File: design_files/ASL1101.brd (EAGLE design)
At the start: 9.8 x 6.5 mm, 4 parts, among them SW1 KMT011

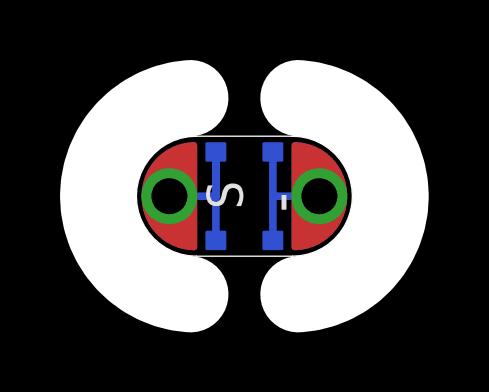
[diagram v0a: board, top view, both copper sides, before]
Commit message: update format
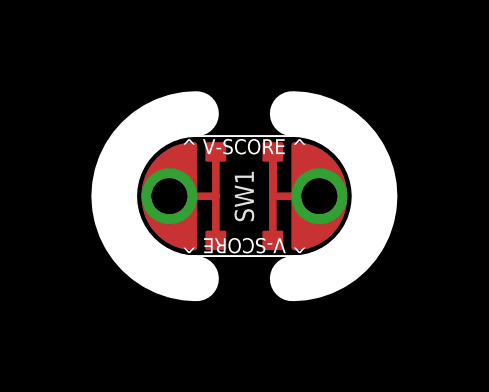
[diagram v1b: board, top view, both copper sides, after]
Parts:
- moved U$1 5.00 mm to (17.5, 20.0), flipped to the bottom
- moved U$7 5.00 mm to (22.5, 20.0), flipped to the bottom
- flipped SW1 to the top
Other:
- board size 9.8 x 6.5 mm -> 8.7 x 5.5 mm
- board text added: "2"
- board text added: "^ V-SCORE ^"
- board text removed: "1"
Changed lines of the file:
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@@
 <?xml version="1.0" encoding="utf-8"?>
 <!DOCTYPE eagle SYSTEM "eagle.dtd">
-<eagle version="6.2">
+<eagle version="6.3">
 <drawing>
 <settings>
@@
 <setting verticaltext="up"/>
 </settings>
-<grid distance="1" unitdist="mil" unit="mm" style="lines" multiple="1" display="yes" altdistance="0.025" altunitdist="inch" altunit="inch"/>
+<grid distance="1" unitdist="mm" unit="mm" style="lines" multiple="1" display="yes" altdistance="0.025" altunitdist="inch" altunit="inch"/>
 <layers>
 <layer number="1" name="Top" color="4" fill="1" visible="yes" active="yes"/>
@@
 <layer number="108" name="Dimension_circle" color="7" fill="1" visible="yes" active="yes"/>
 <layer number="109" name="Dimension_normal" color="7" fill="1" visible="yes" active="yes"/>
+<layer number="110" name="fp0" color="7" fill="1" visible="yes" active="yes"/>
 <layer number="111" name="tGTest" color="4" fill="1" visible="no" active="no"/>
 <layer number="112" name="bGTest" color="1" fill="1" visible="no" active="no"/>
@@
 <layer number="220" name="220bmp" color="7" fill="1" visible="yes" active="yes"/>
 <layer number="221" name="221bmp" color="7" fill="1" visible="yes" active="yes"/>
+<layer number="222" name="222bmp" color="7" fill="1" visible="yes" active="yes"/>
 <layer number="223" name="223bmp" color="7" fill="1" visible="yes" active="yes"/>
 <layer number="224" name="224bmp" color="7" fill="1" visible="yes" active="yes"/>
+<layer number="248" name="Housing" color="7" fill="1" visible="yes" active="yes"/>
+<layer number="249" name="Edge" color="7" fill="1" visible="yes" active="yes"/>
 <layer number="250" name="Descript" color="7" fill="1" visible="yes" active="yes"/>
 <layer number="251" name="SMDround" color="7" fill="1" visible="yes" active="yes"/>
@@
 <text x="48.111025" y="4.365003125" size="0.889" layer="48">TinyLily Switch - 3mm</text>
 <text x="44.986825" y="1.7714" size="0.889" layer="48">AS-PCB-ASL1101</text>
-<text x="67.3810375" y="1.6952" size="0.889" layer="48">1</text>
-<text x="21.884284375" y="19.46078125" size="1.5" layer="21" rot="R90">-</text>
-<text x="19.945059375" y="19.5675375" size="1.2" layer="21" rot="R90">S</text>
+<text x="67.3810375" y="1.6952" size="0.889" layer="48">2</text>
+<text x="18.115715625" y="19.46078125" size="1.5" layer="22" rot="MR90">-</text>
+<text x="20.054940625" y="19.5675375" size="1.2" layer="22" rot="MR90">S</text>
 <dimension x1="18" y1="22" x2="18" y2="18" x3="13.08319375" y3="20" layer="48"/>
 <text x="40.5384" y="14.481796875" size="0.4572" layer="48" ratio="10">Released under the Creative Commons Attribution Share-Alike 3.0 License</text>
@@
 <wire x1="18.4" y1="18" x2="18.4" y2="22" width="0.0254" layer="108" curve="-180"/>
 <wire x1="21.6" y1="22" x2="21.6" y2="18" width="0.0254" layer="108" curve="-180"/>
-<wire x1="18.2" y1="23.27" x2="18.2" y2="16.73" width="2.54" layer="46" curve="173"/>
-<wire x1="21.8" y1="16.73" x2="21.8" y2="23.27" width="2.54" layer="46" curve="173"/>
+<wire x1="18.4" y1="22.75" x2="18.4" y2="17.25" width="1.5" layer="46" curve="180"/>
+<wire x1="21.6" y1="17.25" x2="21.6" y2="22.75" width="1.5" layer="46" curve="180"/>
 <wire x1="18.4" y1="22" x2="21.6" y2="22" width="0.0254" layer="108"/>
 <wire x1="21.6" y1="18" x2="18.4" y2="18" width="0.0254" layer="109"/>
@@
 <wire x1="18.4" y1="22" x2="21.6" y2="22" width="0.0254" layer="20"/>
 <text x="40.5384" y="10.887796875" size="0.4572" layer="48" ratio="10">TinyDuino, TinyLily and TinyShield Designs by TinyCircuits</text>
+<wire x1="16.4" y1="22" x2="23.6" y2="22" width="0.0254" layer="20"/>
+<wire x1="23.6" y1="18" x2="16.4" y2="18" width="0.0254" layer="20"/>
+<text x="20" y="18.6" size="0.5" layer="20" rot="SR180" align="bottom-center">^ V-SCORE ^</text>
+<text x="20" y="21.4" size="0.5" layer="20" rot="SR0" align="bottom-center">^ V-SCORE ^</text>
 </plain>
 <attributes>
@@
 </class>
 </classes>
-<designrules>
+<designrules name="default">
 <description language="de">&lt;b&gt;EAGLE Design Rules&lt;/b&gt;
 &lt;p&gt;
@@
 <attribute name="NO_BOM" value="TRUE" x="44" y="0" size="1.778" layer="27" display="off"/>
 </element>
-<element name="U$1" library="tinycircuits" package="SEWTAP_TH_1206" value="SEWTABTH_1206" x="22.5" y="20" rot="R180">
-<attribute name="BOM" value="EXCLUDE" x="22.5" y="20" size="1.778" layer="27" rot="R180" display="off"/>
-<attribute name="DATABASE" value="./../../../../../Components/TinyCircuits_Part_Database.txt" x="22.5" y="20" size="1.778" layer="27" rot="R180" display="off"/>
-<attribute name="DNP" value="T" x="22.5" y="20" size="1.778" layer="27" rot="R180" display="off"/>
+<element name="U$1" library="tinycircuits" package="SEWTAP_TH_1206" value="SEWTABTH_1206" x="17.5" y="20" rot="MR180">
+<attribute name="BOM" value="EXCLUDE" x="17.5" y="20" size="1.778" layer="28" rot="MR180" display="off"/>
+<attribute name="DATABASE" value="./../../../../../Components/TinyCircuits_Part_Database.txt" x="17.5" y="20" size="1.778" layer="28" rot="MR180" display="off"/>
+<attribute name="DNP" value="T" x="17.5" y="20" size="1.778" layer="28" rot="MR180" display="off"/>
 </element>
-<element name="U$7" library="tinycircuits" package="SEWTAP_TH_1206" value="SEWTABTH_1206" x="17.5" y="20">
-<attribute name="BOM" value="EXCLUDE" x="17.5" y="20" size="1.778" layer="27" display="off"/>
-<attribute name="DATABASE" value="./../../../../../Components/TinyCircuits_Part_Database.txt" x="17.5" y="20" size="1.778" layer="27" display="off"/>
-<attribute name="DNP" value="T" x="17.5" y="20" size="1.778" layer="27" display="off"/>
+<element name="U$7" library="tinycircuits" package="SEWTAP_TH_1206" value="SEWTABTH_1206" x="22.5" y="20" rot="MR0">
+<attribute name="BOM" value="EXCLUDE" x="22.5" y="20" size="1.778" layer="28" rot="MR0" display="off"/>
+<attribute name="DATABASE" value="./../../../../../Components/TinyCircuits_Part_Database.txt" x="22.5" y="20" size="1.778" layer="28" rot="MR0" display="off"/>
+<attribute name="DNP" value="T" x="22.5" y="20" size="1.778" layer="28" rot="MR0" display="off"/>
 </element>
-<element name="SW1" library="tinycircuits" package="KMT011" value="KMT011" x="20" y="20" rot="MR90">
-<attribute name="PARTNO" value="AS-ITM-00041" x="20" y="20" size="1.778" layer="28" rot="MR90" display="off"/>
-<attribute name="VALUE" value="KMT011" x="20" y="20" size="1.778" layer="28" rot="MR90" display="off"/>
+<element name="SW1" library="tinycircuits" package="KMT011" value="KMT011" x="20" y="20" rot="R90">
+<attribute name="PARTNO" value="AS-ITM-00041" x="20" y="20" size="1.778" layer="27" rot="R90" display="off"/>
+<attribute name="VALUE" value="KMT011" x="20" y="20" size="1.778" layer="27" rot="R90" display="off"/>
 </element>
 </elements>
@@
 <contactref element="SW1" pad="4"/>
 <contactref element="SW1" pad="2"/>
-<wire x1="17.5" y1="20" x2="19.05" y2="20" width="0.254" layer="16"/>
-<wire x1="19.05" y1="20" x2="19.05" y2="21.475" width="0.254" layer="16"/>
-<wire x1="19.05" y1="21.475" x2="19.05" y2="18.525" width="0.254" layer="16"/>
+<wire x1="22.5" y1="20" x2="20.95" y2="20" width="0.254" layer="1"/>
+<wire x1="20.95" y1="20" x2="20.95" y2="21.475" width="0.254" layer="1"/>
+<wire x1="20.95" y1="21.475" x2="20.95" y2="18.525" width="0.254" layer="1"/>
 </signal>
 <signal name="-">
@@
 <contactref element="SW1" pad="3"/>
 <contactref element="SW1" pad="1"/>
-<wire x1="20.95" y1="21.475" x2="20.95" y2="20.0152" width="0.254" layer="16"/>
-<wire x1="20.95" y1="20" x2="20.95" y2="18.525" width="0.254" layer="16"/>
-<wire x1="22.5" y1="20" x2="20.95" y2="20" width="0.254" layer="16"/>
-<wire x1="20.95" y1="20" x2="20.95" y2="20.0152" width="0.254" layer="16"/>
+<wire x1="19.05" y1="21.475" x2="19.05" y2="20" width="0.254" layer="1"/>
+<wire x1="19.05" y1="20" x2="19.05" y2="18.525" width="0.254" layer="1"/>
+<wire x1="17.5" y1="20" x2="19.05" y2="20" width="0.254" layer="1"/>
 </signal>
 </signals>
